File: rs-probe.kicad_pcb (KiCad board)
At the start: 4 copper layers, 40 x 14 mm, 97 parts, among them J1 Conn_01x01, J2 Conn_01x01, J3 Conn_01x01, J5 Conn_01x01, J6 Conn_01x01, J7 Conn_01x01, J8 Conn_01x01, J9 Conn_01x01, Q1 NTZD3155C or CMLDM3757-TR-PBF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, SW1 EVQ-P2002W, T1 Tab, T2 Tab, U1 74LVC1T45GM,115, U10 74LVC1T45GM,115, U11 74LVC1T45GM,115, U12 NCP133AMXADJTCG, U13 NCP133AMXADJTCG, U14 NCP133AMXADJTCG, U2 74LVC1T45GM,115, U3 W25Q8, U4 NUF8401MNT4G, U6 RP2040, U7 NUF2042XV6T1G, U8 74LVC1T45GM,115, U9 74LVC1T45GM,115, X1 Conn_ST_STDC14, X10 USB_C_Receptacle_USB2.0

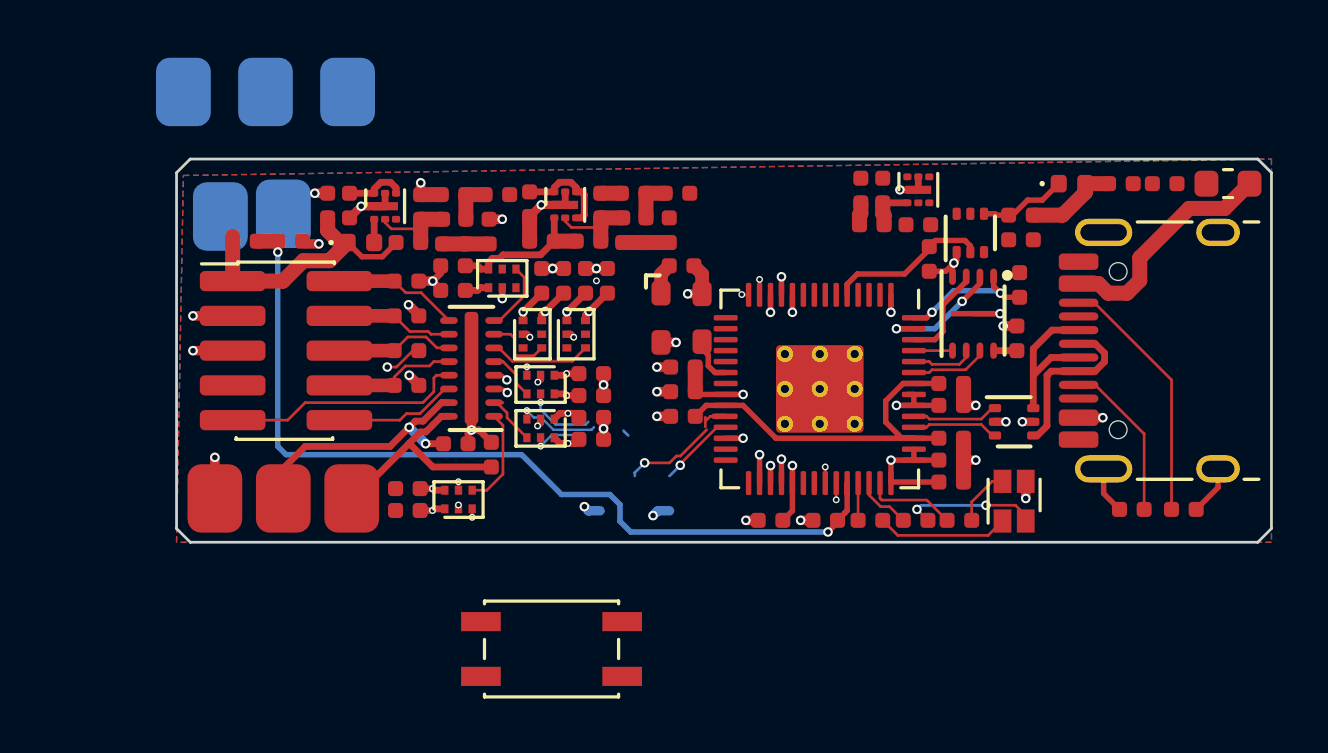
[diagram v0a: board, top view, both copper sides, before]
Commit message: wip
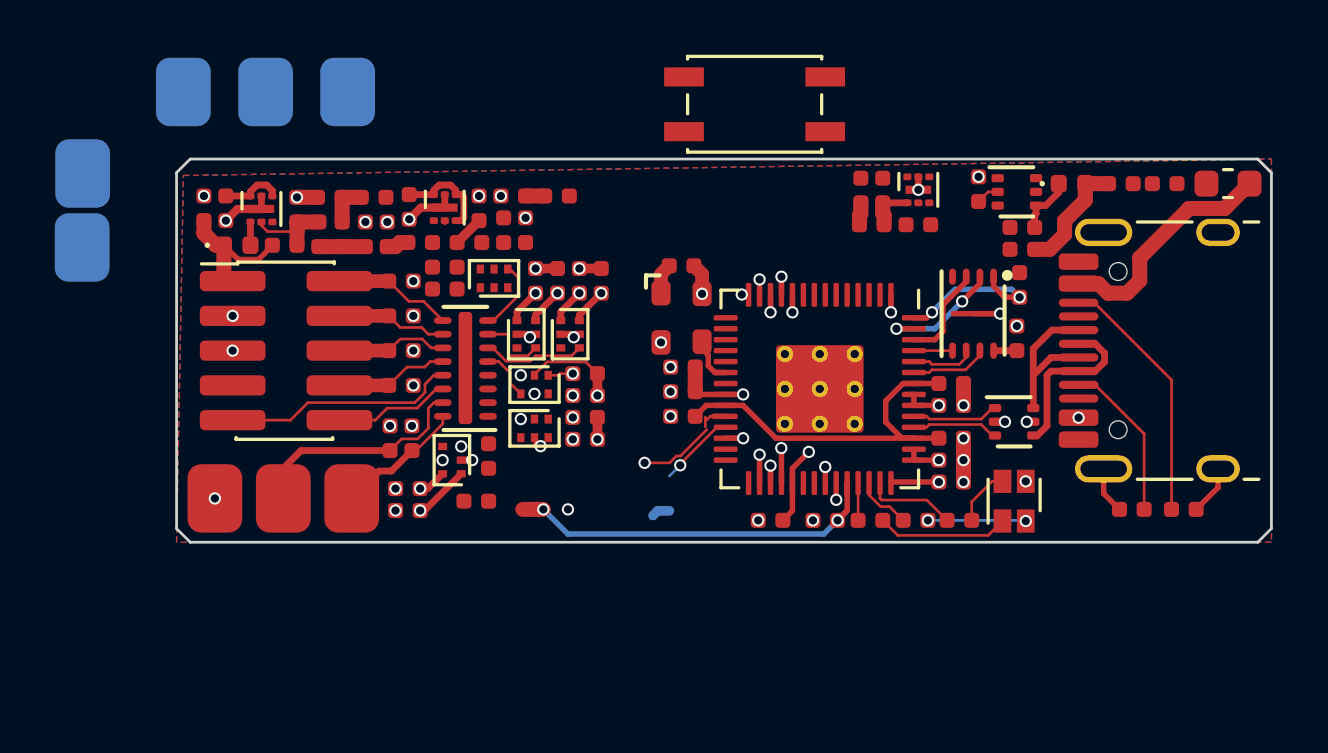
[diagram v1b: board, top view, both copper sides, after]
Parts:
- moved SW1 21.2 mm to (169.6, 77.0)
- moved R9 11.9 mm to (159.9, 89.8), turned to -90 degrees
- moved R11 11.7 mm to (159.4, 91.5), turned to 180 degrees
- moved J6 7.48 mm to (145.1, 79.5)
- moved R12 6.15 mm to (157.4, 82.0)
- moved C21 5.66 mm to (156.2, 81.8), turned to 90 degrees
- moved R27 5.62 mm to (159.2, 82.0), turned to 0 degrees
- moved C28 5.25 mm to (161.2, 81.6)
- moved R29 5.20 mm to (160.4, 81.6)
- moved J5 5.17 mm to (145.1, 82.2)
- moved C27 4.52 mm to (149.5, 80.8)
- moved C5 4.52 mm to (154.1, 80.4)
- moved D3 4.52 mm to (150.7, 82.2)
- moved R1 4.52 mm to (155.7, 80.4)
- moved R14 4.52 mm to (152.4, 82.2)
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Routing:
- net GND: track 41.5 -> 20.1 mm, vias 38 -> 42
- net T_VCC_MEAS: track 32.4 -> 14.1 mm, vias 2 -> 3
- net TRANS_VCC: track 11.2 -> 4.64 mm
- net T_VCC: track 10.0 -> 4.58 mm
- net 5V_KEY_EN: track 5.92 -> 0.84 mm
- net Net-(U1-B): track 3.61 -> 0.00 mm
- net +3.3V: track 27.9 -> 24.5 mm
- net VCP_TX: track 3.72 -> 0.64 mm
- net T_VCP_RX: track 8.15 -> 5.18 mm
- net DIR_TDI: track 2.59 -> 0.00 mm
- net Net-(U2-B): track 2.16 -> 0.00 mm
- net DIR_VCP_TX: track 2.92 -> 0.90 mm
- net ADJ2_T: track 3.17 -> 1.31 mm
- net VS2_T: track 1.60 -> 0.00 mm
- net Net-(D1-RK): track 4.96 -> 3.59 mm
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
